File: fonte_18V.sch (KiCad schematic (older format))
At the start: 35 parts, among them J1 MSTBA, J2 MSTBA, J3 RJ45_Shielded, J4 RJ45_Shielded, Q1 Si2308CDS, U1 LMR16030

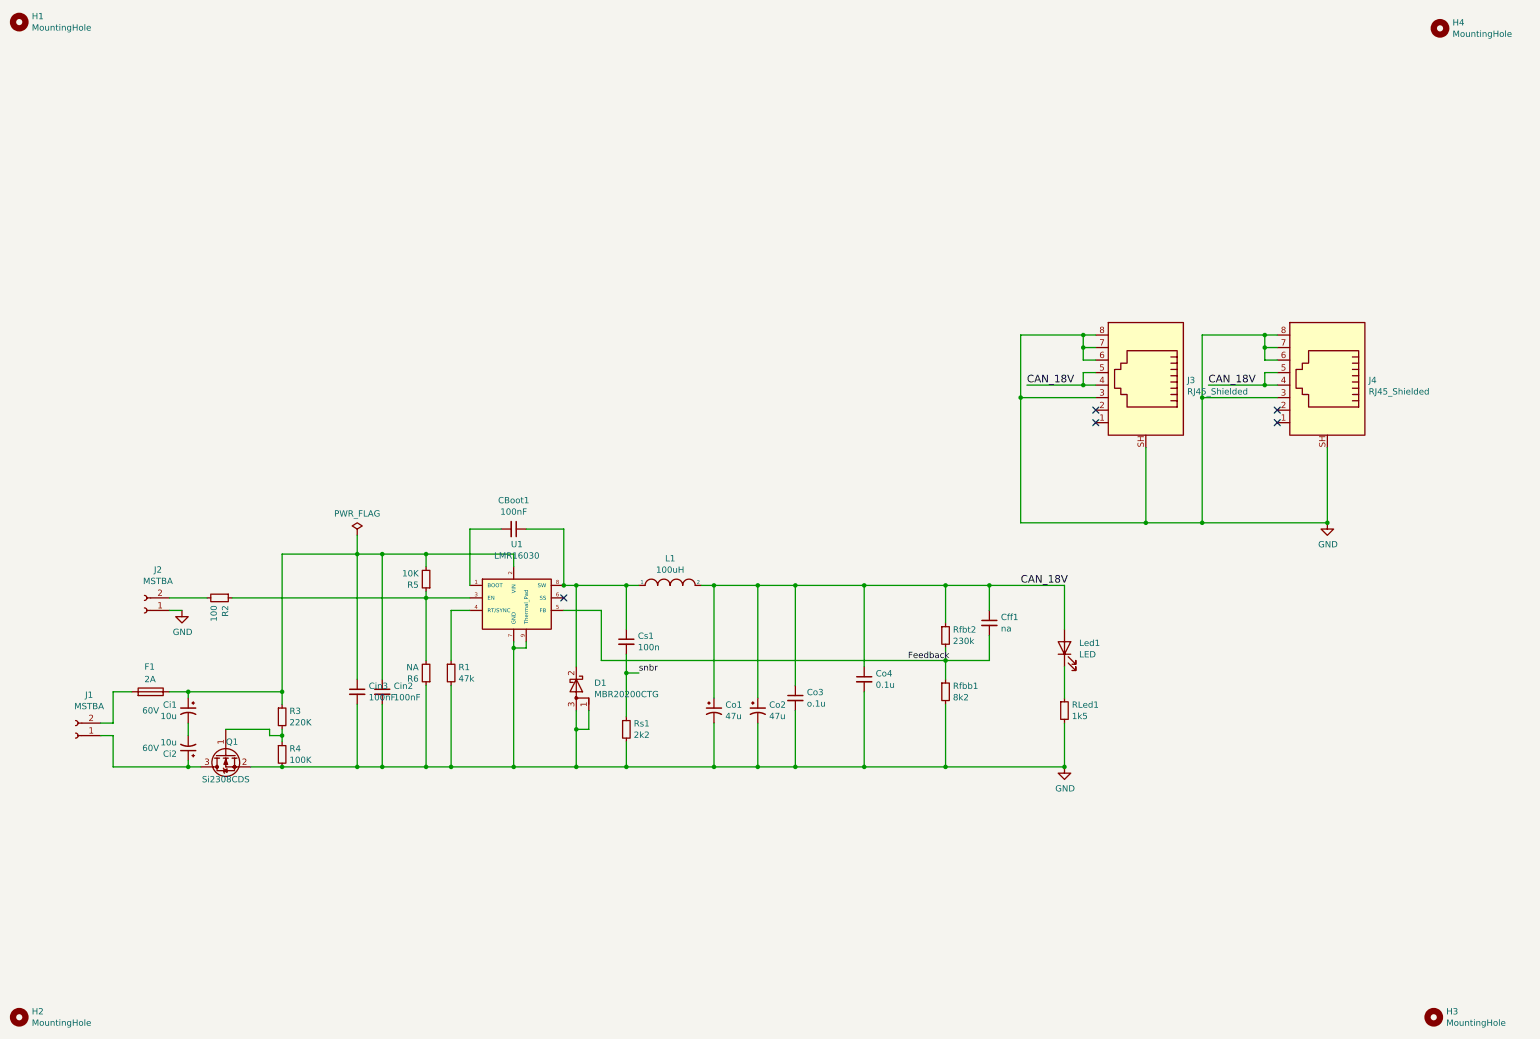
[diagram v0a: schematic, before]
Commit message: atualizado
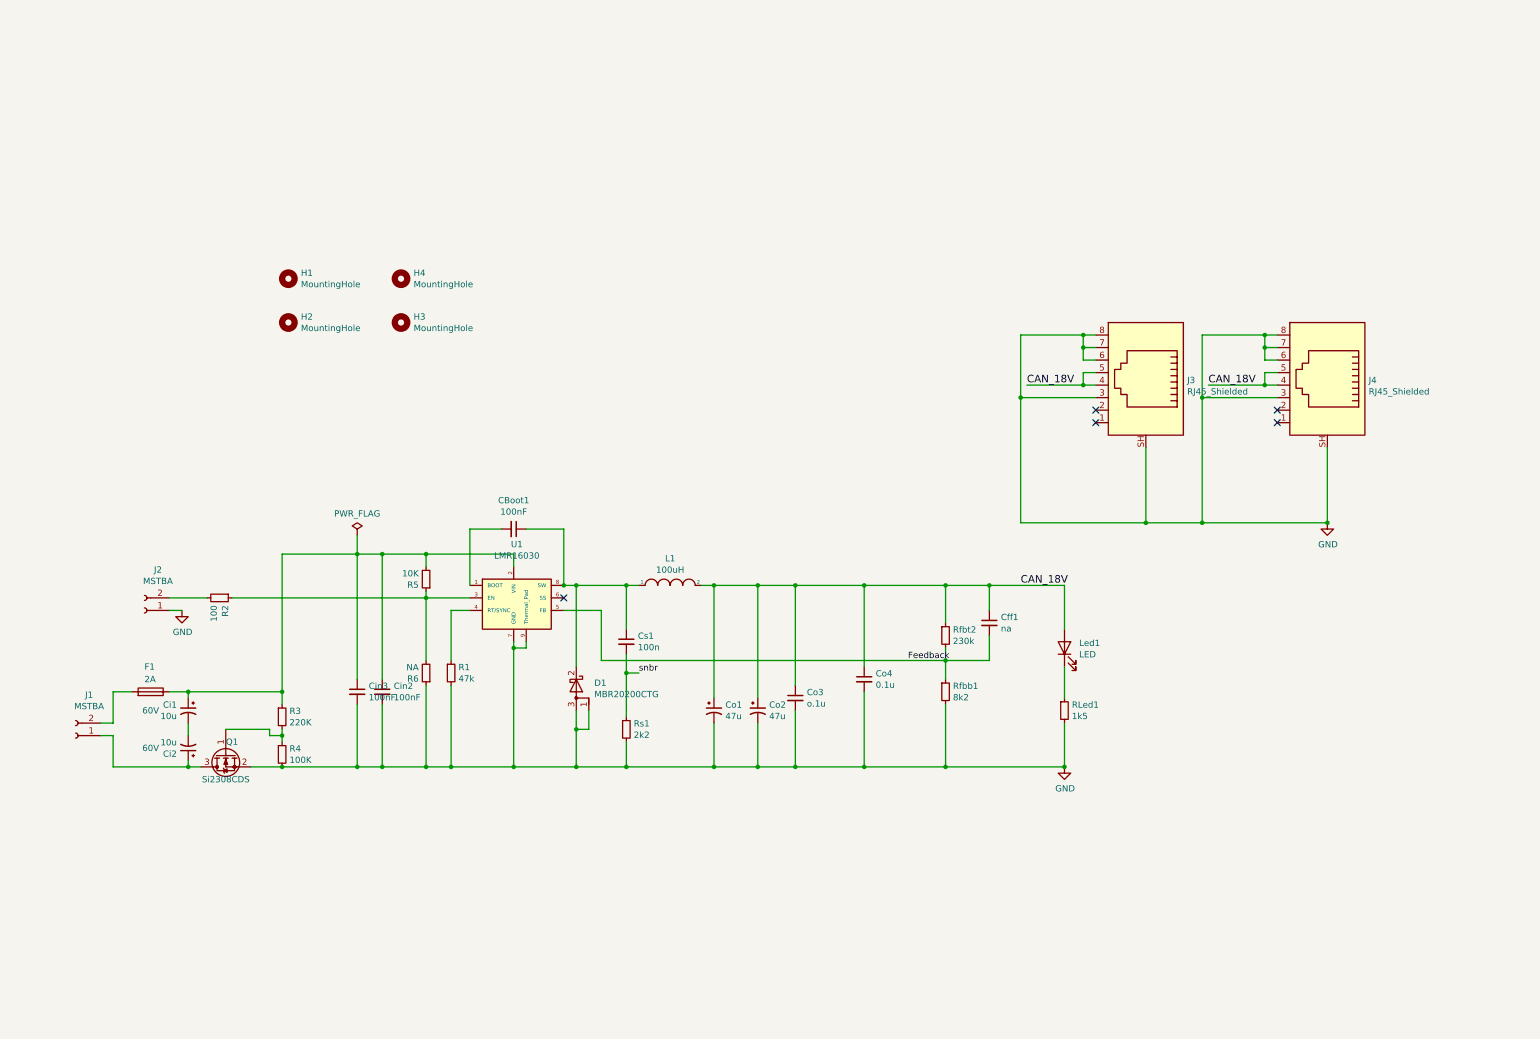
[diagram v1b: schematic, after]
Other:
- moved on the sheet: H1, H2, H3, H4
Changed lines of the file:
@@
 L Mechanical:MountingHole H4
 U 1 1 5DB5A7FD
-P 11550 200
-F 0 "H4" H 11650 246 50  0000 L CNN
-F 1 "MountingHole" H 11650 155 50  0000 L CNN
-F 2 "MountingHole:MountingHole_3.2mm_M3" H 11550 200 50  0001 C CNN
-F 3 "~" H 11550 200 50  0001 C CNN
-	1    11550 200
+P 3250 2200
+F 0 "H4" H 3350 2246 50  0000 L CNN
+F 1 "MountingHole" H 3350 2155 50  0000 L CNN
+F 2 "MountingHole:MountingHole_3.2mm_M3" H 3250 2200 50  0001 C CNN
+F 3 "~" H 3250 2200 50  0001 C CNN
+	1    3250 2200
 	1    0    0    -1
 $EndComp
@@
 L Mechanical:MountingHole H3
 U 1 1 5DB774A1
-P 11500 8100
-F 0 "H3" H 11600 8146 50  0000 L CNN
-F 1 "MountingHole" H 11600 8055 50  0000 L CNN
-F 2 "MountingHole:MountingHole_3.2mm_M3" H 11500 8100 50  0001 C CNN
-F 3 "~" H 11500 8100 50  0001 C CNN
-	1    11500 8100
+P 3250 2550
+F 0 "H3" H 3350 2596 50  0000 L CNN
+F 1 "MountingHole" H 3350 2505 50  0000 L CNN
+F 2 "MountingHole:MountingHole_3.2mm_M3" H 3250 2550 50  0001 C CNN
+F 3 "~" H 3250 2550 50  0001 C CNN
+	1    3250 2550
 	1    0    0    -1
 $EndComp
@@
 L Mechanical:MountingHole H2
 U 1 1 5DB7A851
-P 200 8100
-F 0 "H2" H 300 8146 50  0000 L CNN
-F 1 "MountingHole" H 300 8055 50  0000 L CNN
-F 2 "MountingHole:MountingHole_3.2mm_M3" H 200 8100 50  0001 C CNN
-F 3 "~" H 200 8100 50  0001 C CNN
-	1    200  8100
+P 2350 2550
+F 0 "H2" H 2450 2596 50  0000 L CNN
+F 1 "MountingHole" H 2450 2505 50  0000 L CNN
+F 2 "MountingHole:MountingHole_3.2mm_M3" H 2350 2550 50  0001 C CNN
+F 3 "~" H 2350 2550 50  0001 C CNN
+	1    2350 2550
 	1    0    0    -1
 $EndComp
@@
 L Mechanical:MountingHole H1
 U 1 1 5DB7DBB6
-P 200 150
-F 0 "H1" H 300 196 50  0000 L CNN
-F 1 "MountingHole" H 300 105 50  0000 L CNN
-F 2 "MountingHole:MountingHole_3.2mm_M3" H 200 150 50  0001 C CNN
-F 3 "~" H 200 150 50  0001 C CNN
-	1    200  150
+P 2350 2200
+F 0 "H1" H 2450 2246 50  0000 L CNN
+F 1 "MountingHole" H 2450 2155 50  0000 L CNN
+F 2 "MountingHole:MountingHole_3.2mm_M3" H 2350 2200 50  0001 C CNN
+F 3 "~" H 2350 2200 50  0001 C CNN
+	1    2350 2200
 	1    0    0    -1
 $EndComp
